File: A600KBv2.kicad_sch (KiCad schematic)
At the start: 79 parts, among them J1 32 FFC

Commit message: r2
smaller cutouts for stabilizers in PCB
removed unused mounting holes
board shorter by 2mm top/bottom to mount rails
add 0R option to use capslock under keycap only
silkscreen labels for switches
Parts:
- MX1, MX24: footprint Gateron_KS33_Solderable:Gateron-KS33-Solderable-1.75U -> Amiga Keyboard:Gateron-KS33-Solderable-1.75U
- MX10, MX11, MX14, MX15, MX17, MX20, MX21, MX22, MX23, MX26, MX27, MX28, MX29, MX32, MX33, MX34, MX35, MX38, MX39, MX40, MX41, MX42, MX43, MX47, MX48, MX5, MX50, MX51, MX52, MX53, MX54, MX56, MX57, MX58, MX59, MX6, MX61, MX62, MX63, MX65, MX66, MX67, MX7, MX70, MX72, MX73, MX75, MX76, MX77, MX78, MX8, MX9: footprint Gateron_KS33_Solderable:Gateron-KS33-Solderable-1U -> Amiga Keyboard:Gateron-KS33-Solderable-1U
- MX12, MX13, MX18, MX19, MX2, MX25, MX30, MX31, MX36, MX37, MX46, MX55, MX60, MX64, MX69, MX74: footprint Gateron_KS33_Solderable:Gateron-KS33-Solderable-1.25U -> Amiga Keyboard:Gateron-KS33-Solderable-1.25U
- MX3: footprint Gateron_KS33_Solderable:Gateron-KS33-Solderable-1.5U -> Amiga Keyboard:Gateron-KS33-Solderable-1.5U
- MX4: footprint Amiga_FFC:KS-33-2U-plate-stabilizer -> Amiga Keyboard:Gateron-KS-33-2U-stabilizer
- MX68: footprint Amiga_FFC:KS-33-8_6.25-space-plate-stabilizer -> Amiga Keyboard:KS-33-8U-space
- MX71: footprint Amiga_FFC:KS-33-ISO-plate-stabilizer -> Amiga Keyboard:KS-33-ISO-2U-stabilizer

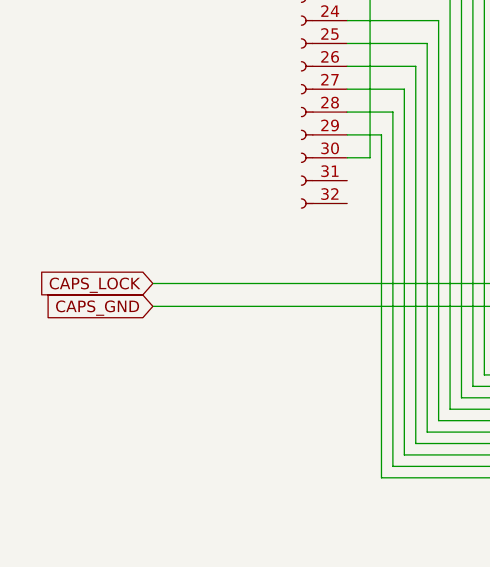
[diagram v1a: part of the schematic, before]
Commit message: fab 9/7/24 KS-33 revised caps LED
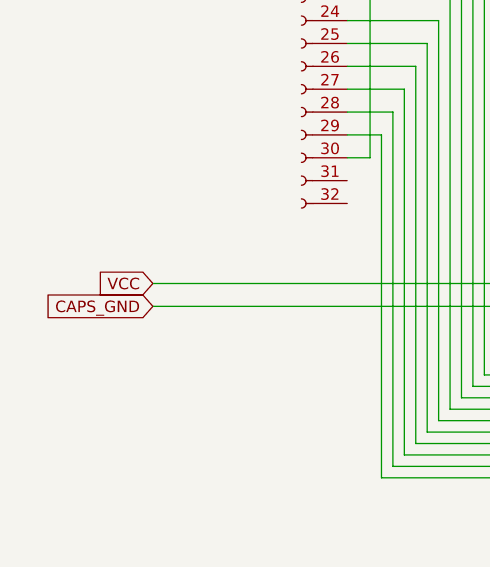
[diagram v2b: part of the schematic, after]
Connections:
- net CAPS_LOCK renamed VCC
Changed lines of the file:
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@@
 		)
 	)
-	(global_label "CAPS_LOCK"
+	(global_label "VCC"
 		(shape input)
 		(at 29.21 133.35 180)
@@
 		)
 		(property "Intersheetrefs" "${INTERSHEET_REFS}"
-			(at 15.5205 133.35 0)
+			(at 22.5962 133.35 0)
 			(effects
 				(font

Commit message: v3
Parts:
- MX68: footprint Amiga Keyboard:KS-33-8U-space -> Amiga Keyboard:KS-33-8-9U-space
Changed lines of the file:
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@@
 			)
 		)
-		(property "Footprint" "Amiga Keyboard:KS-33-8U-space"
+		(property "Footprint" "Amiga Keyboard:KS-33-8-9U-space"
 			(at 235.585 131.445 0)
 			(effects
